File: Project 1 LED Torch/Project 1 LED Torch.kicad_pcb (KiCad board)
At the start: 2 copper layers, 63 x 25 mm, 4 parts, among them SW1 SW_DPDT_x2

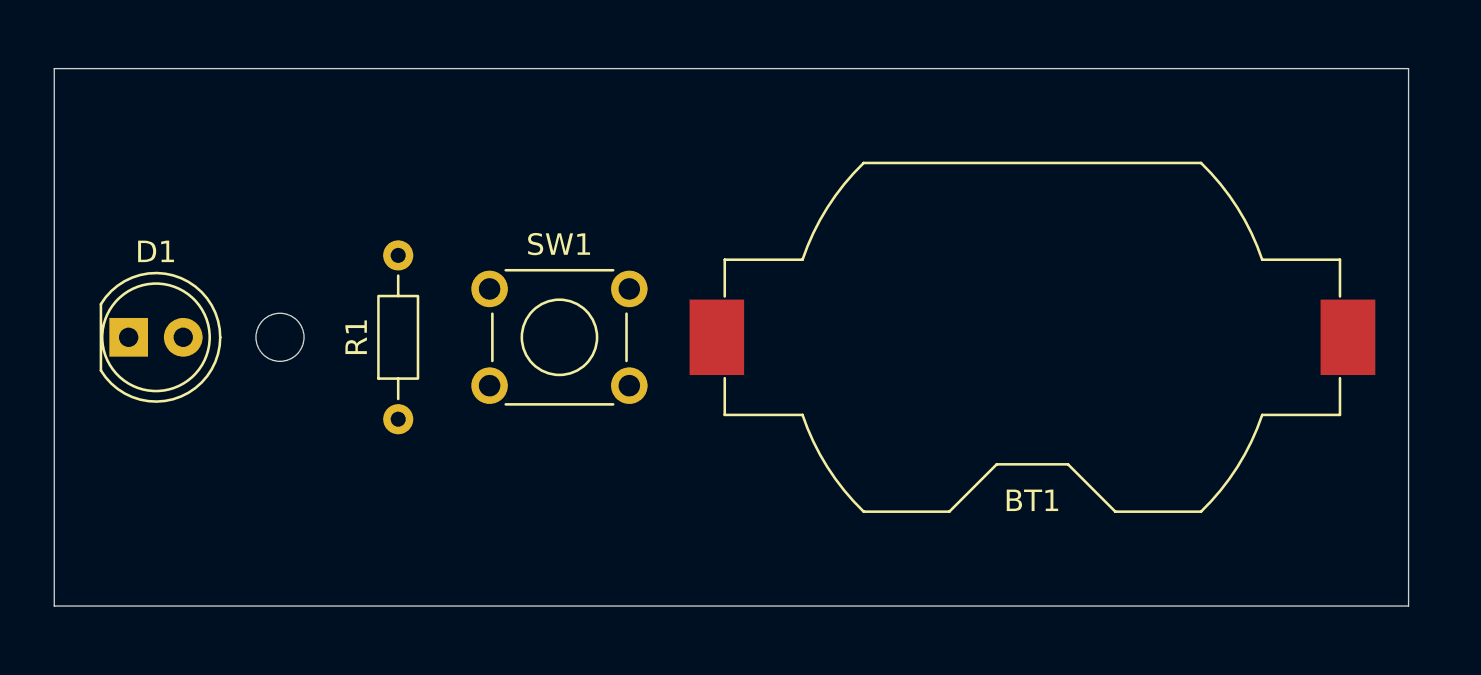
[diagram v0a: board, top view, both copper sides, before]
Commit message: finished PCB design and gerber files from LED torch project
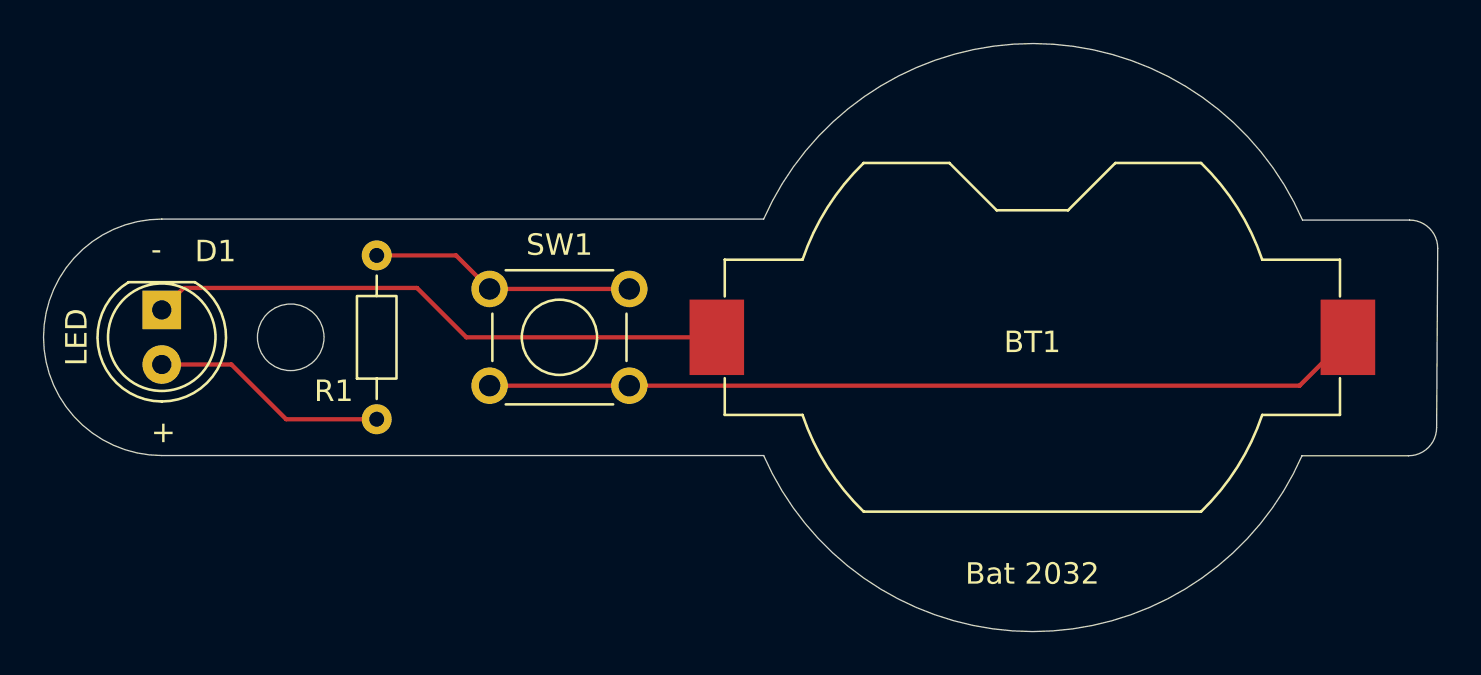
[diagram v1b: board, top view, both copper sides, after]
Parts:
- added REF**: KiCad-Logo2_5mm_SilkScreen, Symbol:KiCad-Logo2_5mm_SilkScreen, B.Cu at (147.5, 121.5)
- BT1: value Battery_Cell -> Bat 2032
- moved D1 2.00 mm to (107.0, 123.7), turned to -90 degrees
- moved R1 1.00 mm to (117.0, 128.8)
- turned BT1 to 180 degrees
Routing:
- net /bat_pos: track 0.00 -> 40.9 mm
- net /LED_cathode: track 0.00 -> 27.2 mm
- net Net-(SW1A-A): track 0.00 -> 12.4 mm
- net /LED_anode: track 0.00 -> 11.1 mm
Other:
- board size 63 x 25 mm -> 64.9 x 27.4 mm
- board text added: "+"
- board text added: "-"
- board text added: "Version 1.0"
